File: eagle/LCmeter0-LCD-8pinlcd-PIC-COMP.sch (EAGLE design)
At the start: 34 parts, among them J1 HD44780-4BIT-8PIN, J2 PIC-UART, J3 PIC-ICSP, J4 J4, J5 CONN-2P-2P, J7 CONN-2P-2P, K2 DS2Y, Q1 20MHz, T1 BC547CBE-A

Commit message: ...
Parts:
- C1, C2: device c:C050-020X036 -> c:C025-025X060
- C3, C4: device c:CPOLE2,5-4 -> c:CPOLE2.5-5
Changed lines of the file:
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@@
 <part name="R4" library="r" deviceset="R" device="0202/7" value="47kΩ"/>
 <part name="R10" library="r" deviceset="R" device="0202/7" value="4.7kΩ"/>
-<part name="C1" library="c" deviceset="C" device="050-020X036" value="1nF"/>
-<part name="C2" library="c" deviceset="C" device="050-020X036" value="1nF"/>
-<part name="C3" library="c" deviceset="CPOL" device="E2,5-4" value="10μF"/>
-<part name="C4" library="c" deviceset="CPOL" device="E2,5-4" value="10μF"/>
+<part name="C1" library="c" deviceset="C" device="025-025X060" value="1nF"/>
+<part name="C2" library="c" deviceset="C" device="025-025X060" value="1nF"/>
+<part name="C3" library="c" deviceset="CPOL" device="E2.5-5" value="10μF"/>
+<part name="C4" library="c" deviceset="CPOL" device="E2.5-5" value="10μF"/>
 <part name="C5" library="c" deviceset="C" device="025-020X036" value="33pF"/>
 <part name="C6" library="c" deviceset="C" device="025-020X036" value="33pF"/>

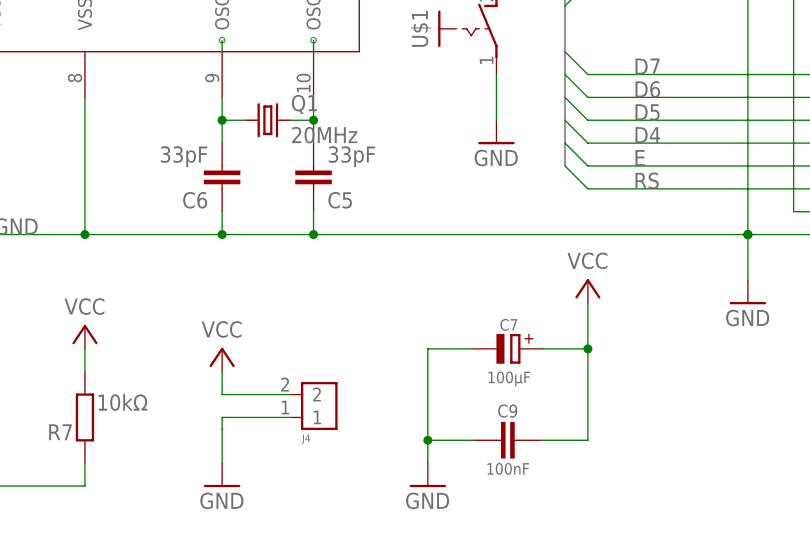
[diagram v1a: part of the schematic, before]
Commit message: ...
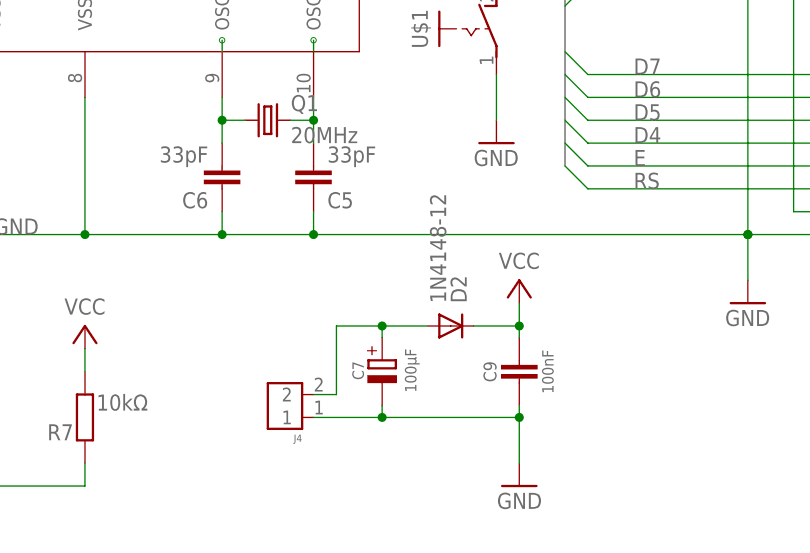
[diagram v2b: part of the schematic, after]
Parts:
- added D2: 1N4148-12, d:1N4148-12
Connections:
- new net N$12: C7.+, D2.A, J4.2
- net VCC: now also D2.C; no longer C7.+, J4.2
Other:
- moved on the sheet: C7, C9, J4
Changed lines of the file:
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@@
 <part name="C9" library="rcl" deviceset="C-EU" device="025-024X044" value="100nF"/>
 <part name="GND2" library="supply1" deviceset="GND" device=""/>
-<part name="GND4" library="supply1" deviceset="GND" device=""/>
 <part name="GND5" library="supply1" deviceset="GND" device=""/>
 <part name="GND6" library="supply1" deviceset="GND" device=""/>
@@
 <part name="LED1" library="led" deviceset="TLLG4400" device=""/>
 <part name="GND10" library="supply1" deviceset="GND" device=""/>
-<part name="P+8" library="supply1" deviceset="VCC" device=""/>
 <part name="GND13" library="supply1" deviceset="GND" device=""/>
 <part name="J4" library="pinconn" deviceset="CONN-2P" device="-2P" value="J4"/>
@@
 <part name="J7" library="pinconn" deviceset="CONN-2P" device="-2P"/>
 <part name="J5" library="pinconn" deviceset="CONN-2P" device="-2P"/>
+<part name="D2" library="d" deviceset="1N4148" device="-12" value="1N4148-12"/>
 </parts>
 <sheets>
@@
 <instance part="C5" gate="G$1" x="177.8" y="-2.54" rot="MR180"/>
 <instance part="C6" gate="G$1" x="167.64" y="-2.54" rot="R180"/>
-<instance part="C7" gate="G$1" x="199.39" y="-20.32" smashed="yes" rot="R270">
-<attribute name="NAME" x="199.517" y="-18.288" size="1.27" layer="95" rot="R180" align="top-center"/>
-<attribute name="VALUE" x="199.517" y="-22.86" size="1.27" layer="96" rot="R180" align="bottom-center"/>
-</instance>
-<instance part="C9" gate="G$1" x="200.66" y="-30.48" smashed="yes" rot="R270">
-<attribute name="NAME" x="199.39" y="-27.94" size="1.4224" layer="95" align="bottom-center"/>
-<attribute name="VALUE" x="199.39" y="-33.02" size="1.27" layer="96" align="top-center"/>
+<instance part="C7" gate="G$1" x="185.42" y="-22.86" smashed="yes">
+<attribute name="NAME" x="183.388" y="-22.733" size="1.27" layer="95" rot="R270" align="top-center"/>
+<attribute name="VALUE" x="187.96" y="-22.733" size="1.27" layer="96" rot="R270" align="bottom-center"/>
+</instance>
+<instance part="C9" gate="G$1" x="200.66" y="-21.59" smashed="yes">
+<attribute name="NAME" x="198.12" y="-22.86" size="1.4224" layer="95" rot="R90" align="bottom-center"/>
+<attribute name="VALUE" x="203.2" y="-22.86" size="1.27" layer="96" rot="R90" align="top-center"/>
 </instance>
 <instance part="GND2" gate="1" x="58.42" y="5.08"/>
-<instance part="GND4" gate="1" x="190.5" y="-35.56"/>
 <instance part="GND5" gate="1" x="22.86" y="-2.54"/>
 <instance part="GND6" gate="1" x="35.56" y="-2.54"/>
@@
 <instance part="L1" gate="G$1" x="12.7" y="25.4" rot="R90"/>
 <instance part="Q1" gate="G$1" x="172.72" y="5.08"/>
-<instance part="P+3" gate="VCC" x="208.28" y="-12.7" smashed="yes">
-<attribute name="VALUE" x="208.28" y="-11.43" size="1.778" layer="96" align="bottom-center"/>
+<instance part="P+3" gate="VCC" x="200.66" y="-12.7" smashed="yes">
+<attribute name="VALUE" x="200.66" y="-11.43" size="1.778" layer="96" align="bottom-center"/>
 </instance>
 <instance part="P+4" gate="VCC" x="43.18" y="63.5" smashed="yes">
@@
 <instance part="LED1" gate="G$1" x="72.39" y="0" rot="MR90"/>
 <instance part="GND10" gate="1" x="66.04" y="-5.08"/>
-<instance part="P+8" gate="VCC" x="167.64" y="-20.32" smashed="yes">
-<attribute name="VALUE" x="167.64" y="-19.05" size="1.778" layer="96" align="bottom-center"/>
-</instance>
-<instance part="GND13" gate="1" x="167.64" y="-35.56"/>
-<instance part="J4" gate="G$1" x="177.8" y="-27.94"/>
+<instance part="GND13" gate="1" x="200.66" y="-35.56" rot="MR0"/>
+<instance part="J4" gate="G$1" x="175.26" y="-27.94" rot="MR0"/>
 <instance part="J2" gate="1" x="134.62" y="-11.43"/>
 <instance part="GND15" gate="1" x="121.92" y="-21.59"/>
@@
 <instance part="J7" gate="G$1" x="-22.86" y="25.4" rot="MR0"/>
 <instance part="J5" gate="G$1" x="-22.86" y="0" rot="MR0"/>
+<instance part="D2" gate="G$1" x="193.04" y="-17.78" rot="R270"/>
 </instances>
 <busses>
@@
 <pinref part="GND2" gate="1" pin="GND"/>
 <wire x1="58.42" y1="10.16" x2="58.42" y2="7.62" width="0.1524" layer="91"/>
-</segment>
-<segment>
-<pinref part="GND4" gate="1" pin="GND"/>
-<pinref part="C7" gate="G$1" pin="-"/>
-<pinref part="C9" gate="G$1" pin="2"/>
-<wire x1="190.5" y1="-30.48" x2="190.5" y2="-20.32" width="0.1524" layer="91"/>
-<wire x1="190.5" y1="-20.32" x2="195.58" y2="-20.32" width="0.1524" layer="91"/>
-<wire x1="190.5" y1="-33.02" x2="190.5" y2="-30.48" width="0.1524" layer="91"/>
-<wire x1="190.5" y1="-30.48" x2="195.58" y2="-30.48" width="0.1524" layer="91"/>
-<junction x="190.5" y="-30.48"/>
 </segment>
 <segment>
@@
 <segment>
 <pinref part="GND13" gate="1" pin="GND"/>
-<wire x1="167.64" y1="-33.02" x2="167.64" y2="-29.21" width="0.1524" layer="91"/>
+<wire x1="200.66" y1="-33.02" x2="200.66" y2="-27.94" width="0.1524" layer="91"/>
 <pinref part="J4" gate="G$1" pin="1"/>
-<wire x1="175.26" y1="-27.94" x2="167.64" y2="-27.94" width="0.1524" layer="91"/>
-<wire x1="167.64" y1="-27.94" x2="167.64" y2="-29.21" width="0.1524" layer="91"/>
+<wire x1="200.66" y1="-27.94" x2="185.42" y2="-27.94" width="0.1524" layer="91"/>
+<wire x1="177.8" y1="-27.94" x2="185.42" y2="-27.94" width="0.1524" layer="91"/>
+<wire x1="185.42" y1="-27.94" x2="185.42" y2="-26.67" width="0.1524" layer="91"/>
+<pinref part="C7" gate="G$1" pin="-"/>
+<junction x="185.42" y="-27.94"/>
+<pinref part="C9" gate="G$1" pin="2"/>
+<wire x1="200.66" y1="-26.67" x2="200.66" y2="-27.94" width="0.1524" layer="91"/>
+<junction x="200.66" y="-27.94"/>
 </segment>
 <segment>
@@
 <pinref part="P+5" gate="VCC" pin="VCC"/>
 <wire x1="124.46" y1="55.88" x2="124.46" y2="58.42" width="0.1524" layer="91"/>
-</segment>
-<segment>
-<pinref part="C7" gate="G$1" pin="+"/>
-<pinref part="C9" gate="G$1" pin="1"/>
-<wire x1="203.2" y1="-20.32" x2="208.28" y2="-20.32" width="0.1524" layer="91"/>
-<wire x1="208.28" y1="-20.32" x2="208.28" y2="-30.48" width="0.1524" layer="91"/>
-<wire x1="208.28" y1="-30.48" x2="203.2" y2="-30.48" width="0.1524" layer="91"/>
-<pinref part="P+3" gate="VCC" pin="VCC"/>
-<wire x1="208.28" y1="-20.32" x2="208.28" y2="-15.24" width="0.1524" layer="91"/>
-<junction x="208.28" y="-20.32"/>
 </segment>
 <segment>
@@
 </segment>
 <segment>
-<pinref part="P+8" gate="VCC" pin="VCC"/>
-<wire x1="167.64" y1="-25.4" x2="167.64" y2="-22.86" width="0.1524" layer="91"/>
-<pinref part="J4" gate="G$1" pin="2"/>
-<wire x1="167.64" y1="-25.4" x2="175.26" y2="-25.4" width="0.1524" layer="91"/>
-</segment>
-<segment>
 <pinref part="J2" gate="1" pin="VDD"/>
 <pinref part="P+9" gate="VCC" pin="VCC"/>
@@
 <wire x1="132.08" y1="58.42" x2="132.08" y2="43.18" width="0.1524" layer="91"/>
 <pinref part="U$2" gate="G$1" pin="VDD"/>
+</segment>
+<segment>
+<pinref part="D2" gate="G$1" pin="C"/>
+<wire x1="195.58" y1="-17.78" x2="200.66" y2="-17.78" width="0.1524" layer="91"/>
+<wire x1="200.66" y1="-17.78" x2="200.66" y2="-15.24" width="0.1524" layer="91"/>
+<pinref part="P+3" gate="VCC" pin="VCC"/>
+<pinref part="C9" gate="G$1" pin="1"/>
+<wire x1="200.66" y1="-19.05" x2="200.66" y2="-17.78" width="0.1524" layer="91"/>
+<junction x="200.66" y="-17.78"/>
 </segment>
 </net>
@@
 </segment>
 </net>
+<net name="N$12" class="0">
+<segment>
+<wire x1="180.34" y1="-17.78" x2="185.42" y2="-17.78" width="0.1524" layer="91"/>
+<pinref part="J4" gate="G$1" pin="2"/>
+<wire x1="185.42" y1="-17.78" x2="190.5" y2="-17.78" width="0.1524" layer="91"/>
+<wire x1="180.34" y1="-17.78" x2="180.34" y2="-25.4" width="0.1524" layer="91"/>
+<wire x1="180.34" y1="-25.4" x2="177.8" y2="-25.4" width="0.1524" layer="91"/>
+<pinref part="C7" gate="G$1" pin="+"/>
+<wire x1="185.42" y1="-19.05" x2="185.42" y2="-17.78" width="0.1524" layer="91"/>
+<junction x="185.42" y="-17.78"/>
+<pinref part="D2" gate="G$1" pin="A"/>
+</segment>
+</net>

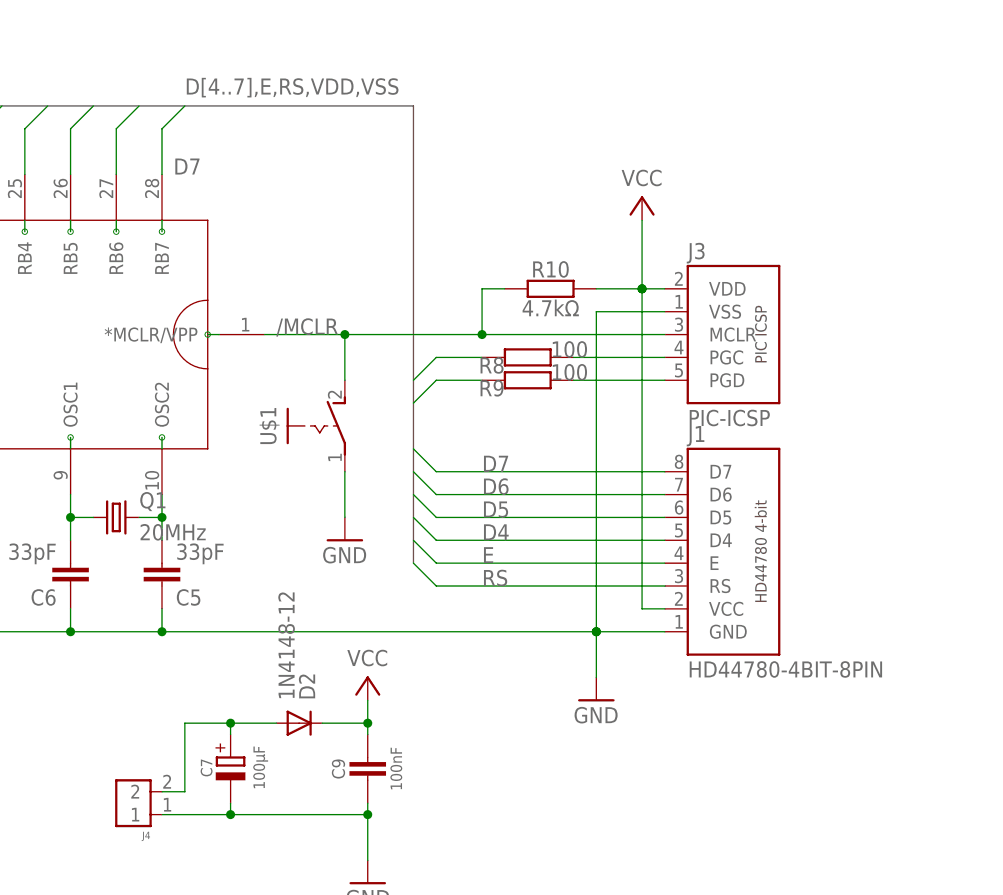
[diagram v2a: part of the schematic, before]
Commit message: ...
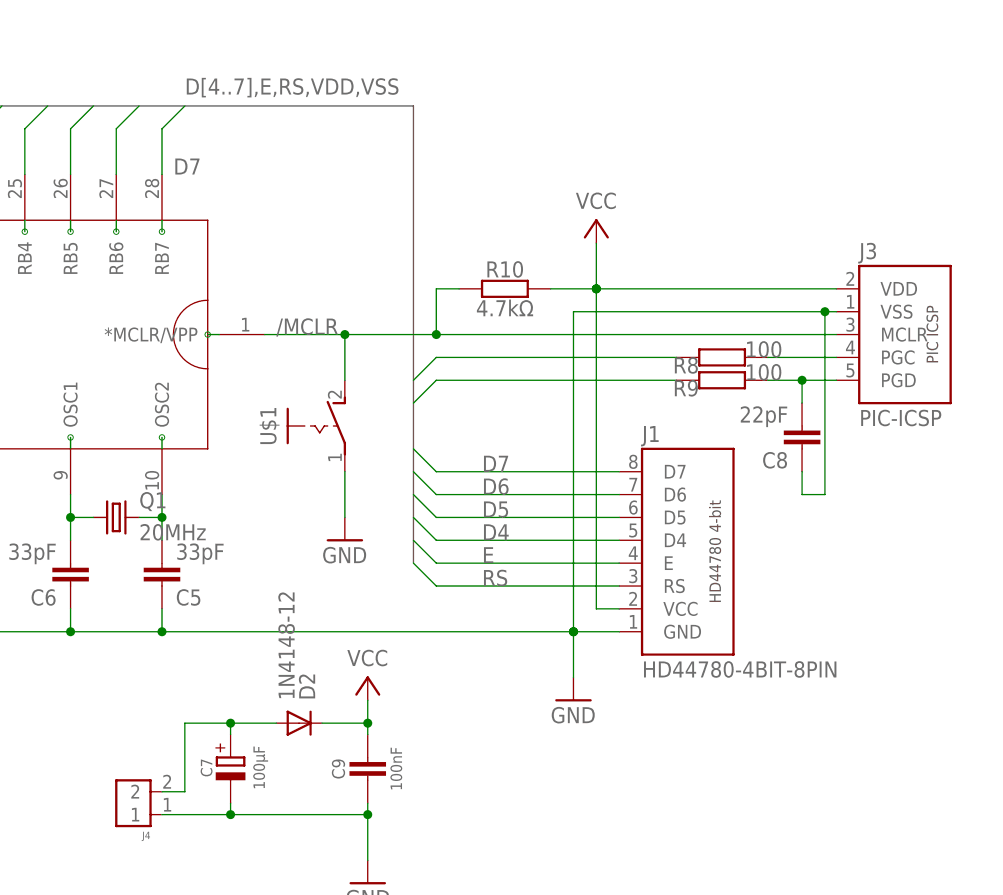
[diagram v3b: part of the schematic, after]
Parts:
- added C8: 22pF, c:C050-020X036
- C7: device c:CPOLE2.5-6 -> c:CPOLE2.5-5
- R8: device r:R0202/5 -> r:R0202/7
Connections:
- net N$1 renamed PGC
- removed net N$3: J3.PGD, R9.1
- new net PGD: C8.2, J3.PGD, R9.1
- net D6: now also R8.2; no longer R9.2
- net D7: now also R9.2; no longer R8.2
- net GND: now also C8.1
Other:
- moved on the sheet: J1, J3, R10, R8, R9
